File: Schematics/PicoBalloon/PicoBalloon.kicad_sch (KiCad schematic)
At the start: 32 parts, among them J1 ANT, J2 SOLAR_L, J3 SOLAR_R, J4 GPS_ANT, J5 SWD, Q1 IRLM2502, U1 STM32F103C8Tx, U2 MCP1640Bx-xCHY, U3 TMP20AIDCK

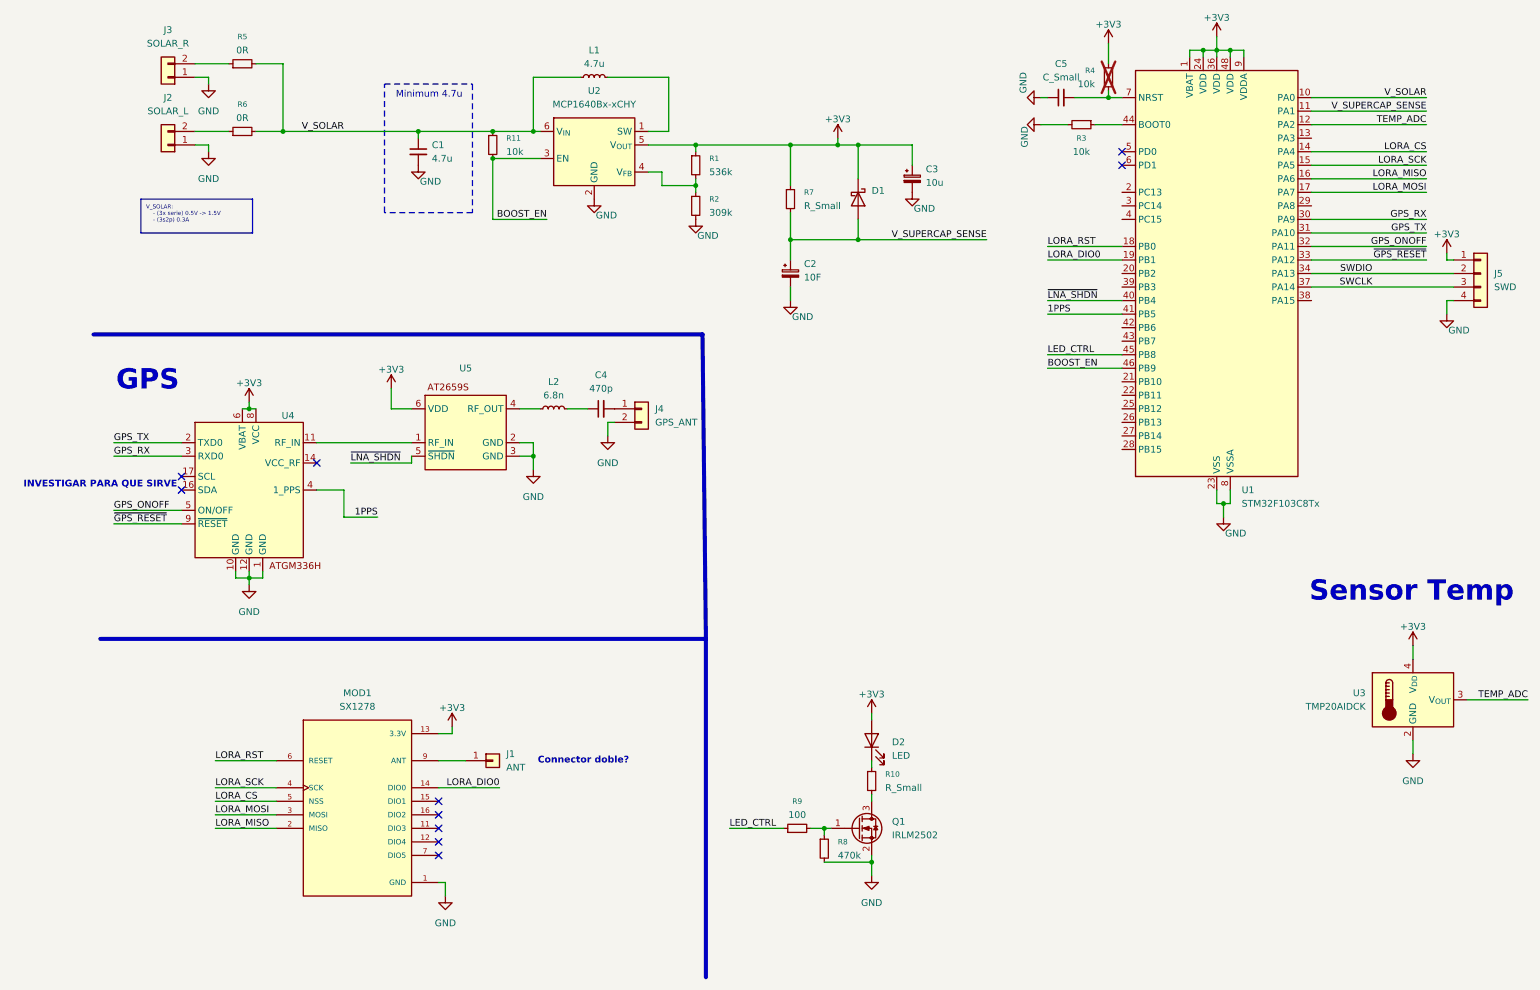
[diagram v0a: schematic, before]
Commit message: Finished schematic V1
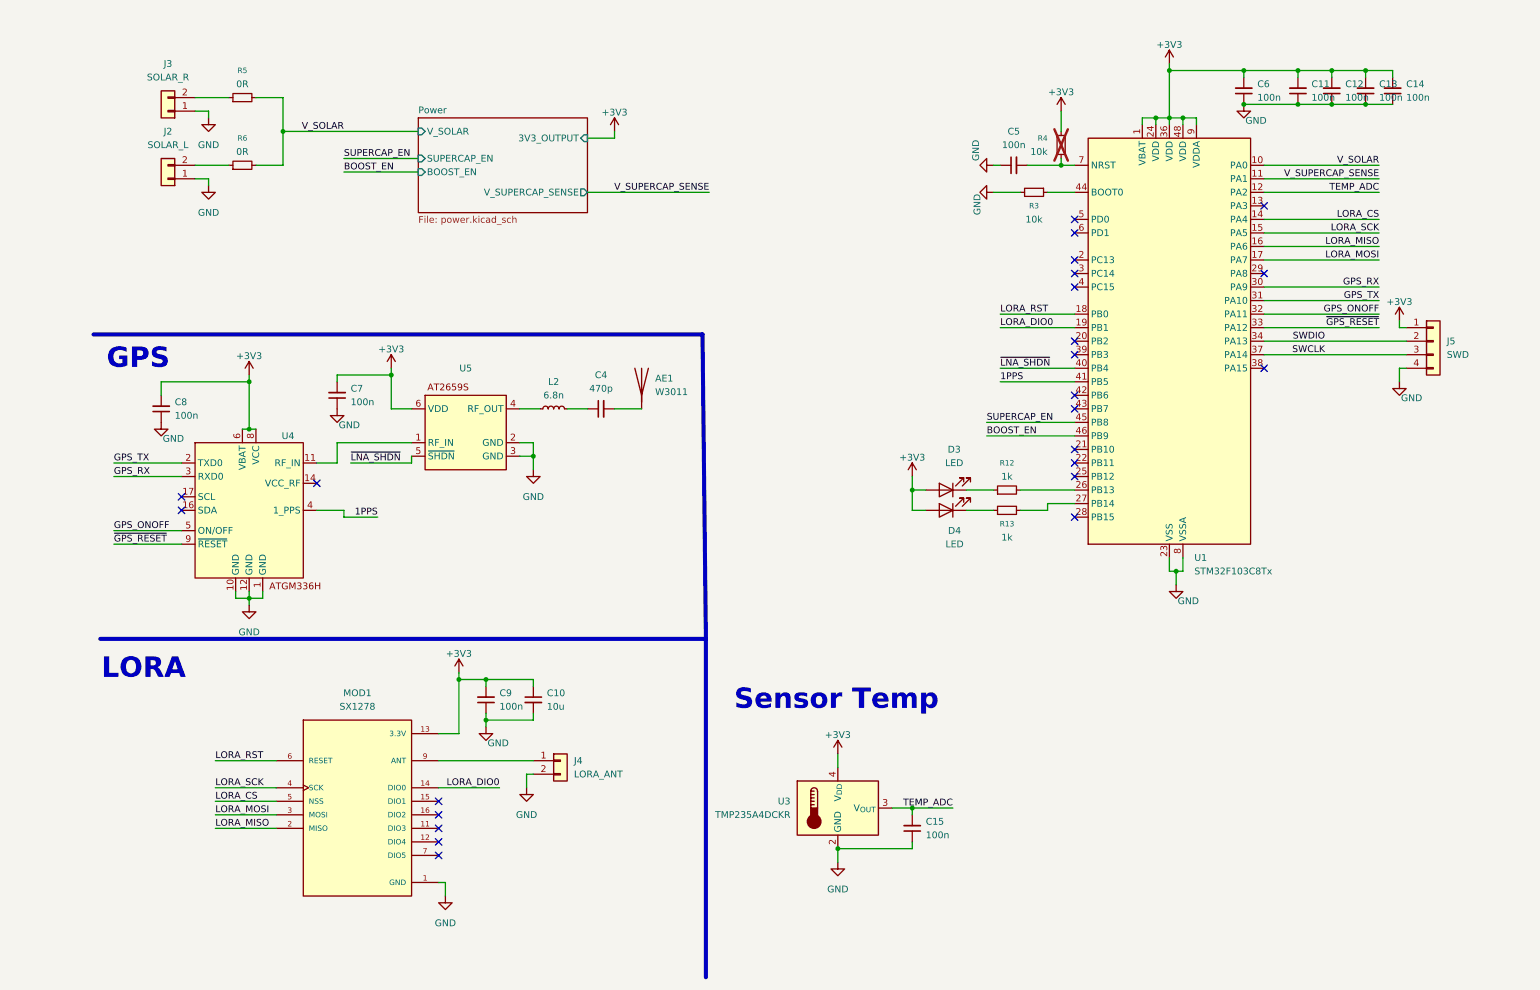
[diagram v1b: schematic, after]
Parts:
- removed C1: 4.7u, symbol Device:C_Small
- removed C2: 10F, symbol Device:C_Polarized_Small
- removed C3: 10u, symbol Device:C_Polarized_Small
- removed D1: D_Schottky, symbol Device:D_Schottky
- removed D2: LED, symbol Device:LED
- removed J1: ANT, symbol Connector_Generic:Conn_01x01
- removed L1: 4.7u, Inductor_SMD:L_1008_2520Metric_Pad1.43x2.20mm_HandSolder, symbol Device:L_Small
- removed Q1: IRLM2502, Package_TO_SOT_SMD:SOT-23_Handsoldering, symbol Transistor_FET:Q_NMOS_GSD
- removed R1: 536k, Resistor_SMD:R_0805_2012Metric_Pad1.20x1.40mm_HandSolder, symbol Device:R_Small
- removed R10, R7: R_Small, symbol Device:R_Small
- removed R11: 10k, symbol Device:R_Small
- removed R2: 309k, Resistor_SMD:R_0805_2012Metric_Pad1.20x1.40mm_HandSolder, symbol Device:R_Small
- removed R8: 470k, symbol Device:R_Small
- removed R9: 100, symbol Device:R_Small
- removed U2: MCP1640Bx-xCHY, Package_TO_SOT_SMD:SOT-23-6, symbol Regulator_Switching:MCP1640Cx-xCHY
- added AE1: W3011, RF_Antenna:Pulse_W3011, symbol Device:Antenna
- added C10: 10u, Capacitor_SMD:C_0805_2012Metric_Pad1.18x1.45mm_HandSolder, symbol Device:C_Small
- added C11, C12, C13, C14, C15, C6, C7, C8, C9: 100n, Capacitor_SMD:C_0603_1608Metric_Pad1.08x0.95mm_HandSolder, symbol Device:C_Small
- added D3, D4: LED, LED_SMD:LED_0603_1608Metric_Pad1.05x0.95mm_HandSolder, symbol Device:LED
- added R12, R13: 1k, Resistor_SMD:R_0603_1608Metric_Pad0.98x0.95mm_HandSolder, symbol Device:R_Small
- C4: footprint (none) -> Capacitor_SMD:C_0603_1608Metric_Pad1.08x0.95mm_HandSolder; LCSC (none) -> https://lcsc.com/product-detail/Multilayer-Ceramic-Capacito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
- C5: value C_Small -> 100n; footprint (none) -> Capacitor_SMD:C_0603_1608Metric_Pad1.08x0.95mm_HandSolder; LCSC (none) -> https://lcsc.com/product-detail/Multilayer-Ceramic-Capacito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
- J2, J3: footprint (none) -> Connector_PinHeader_2.00mm:PinHeader_1x02_P2.00mm_Vertical
- J4: value GPS_ANT -> LORA_ANT; footprint (none) -> Connector_PinHeader_2.00mm:PinHeader_1x02_P2.00mm_Vertical
- J5: footprint (none) -> Connector_PinHeader_2.54mm:PinHeader_1x04_P2.54mm_Vertical
- L2: footprint Inductor_SMD:L_0805_2012Metric_Pad1.05x1.20mm_HandSolder -> Inductor_SMD:L_0603_1608Metric_Pad1.05x0.95mm_HandSolder; LCSC https://lcsc.com/product-detail/Inductors-SMD_FH-VHF201209H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 -> https://lcsc.com/product-detail/Inductors-SMD_HYHONGYEX-HBL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
- R3, R4, R5, R6: footprint (none) -> Resistor_SMD:R_0603_1608Metric_Pad0.98x0.95mm_HandSolder
- U3: value TMP20AIDCK -> TMP235A4DCKR; LCSC (none) -> https://lcsc.com/product-detail/Temperature-Sensors_TI-TMP2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
- U5: LCSC (none) -> https://lcsc.com/product-detail/Low-Noise-Amplifiers-LNA-RF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
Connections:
- net +3V3: now also C10.1, C11.2, C12.2, C13.2, C14.2, C6.2, C7.2, C8.2, C9.2, D3.2 (A), D4.2 (A)
- net GND: now also C10.2, C11.1, C12.1, C13.1, C14.1, C15.1, C6.1, C7.1, C8.1, C9.1
- net TEMP_ADC: now also C15.2
- net at MOD1.9 (ANT): now also J4.1 (Pin_1)
- net at C4.2: now also AE1.1 (A); no longer J4.1 (Pin_1)
- net at U1.26 (PB13): now also R12.2
- net at U1.27 (PB14): now also R13.2
- net LED_CTRL renamed SUPERCAP_EN
- new net: D4.1 (K), R13.1
- new net: D3.1 (K), R12.1
- no-connect marks 10 -> 24
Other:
- added sheet Power (power.kicad_sch)
- note added: "LORA"
- note removed: "Connector doble?"
- note removed: "INVESTIGAR PARA QUE SIRVE"
- note removed: "Minimum 4.7u"
- moved on the sheet: C5, J2, J3, J5, R3, R4, R5, R6, U1, U3, U4
